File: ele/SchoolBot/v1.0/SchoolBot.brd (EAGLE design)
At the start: 100.1 x 58.3 mm, 56 parts, among them X1 M8, X2 M8, X4 POWER_IN

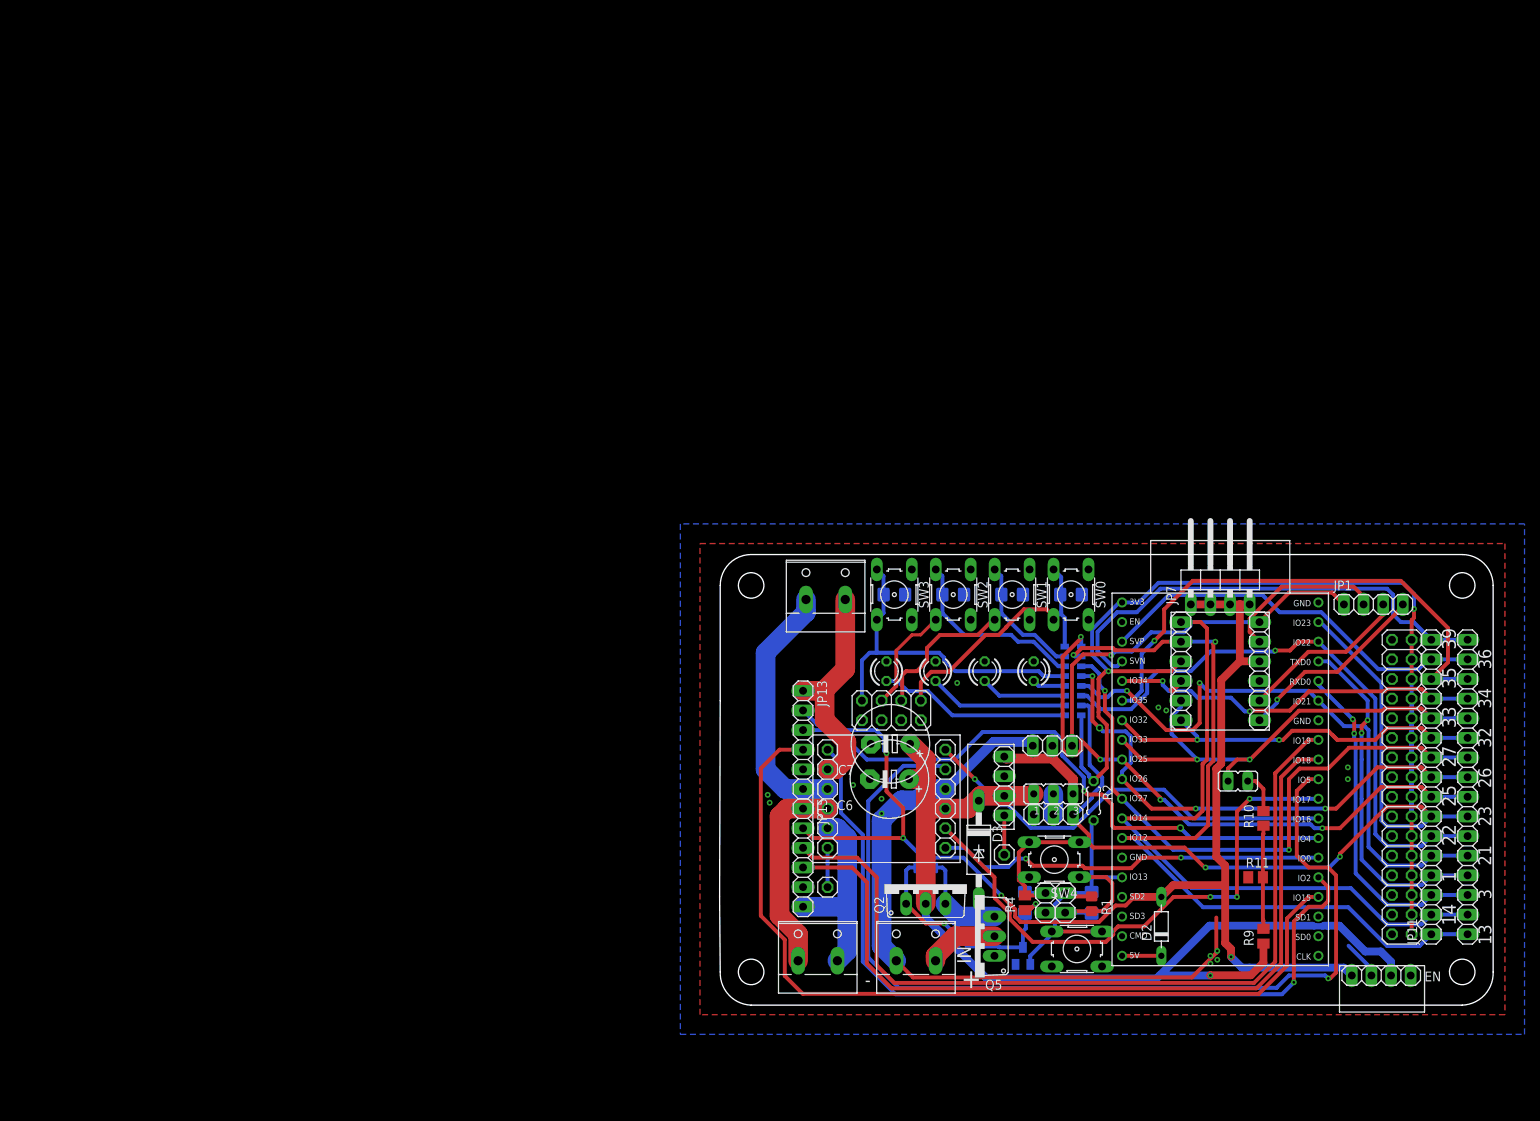
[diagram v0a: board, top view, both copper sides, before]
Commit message: new board
-komplenti prekreslini desky
-doplneni rady pinhedu gnd pro 5v piniste
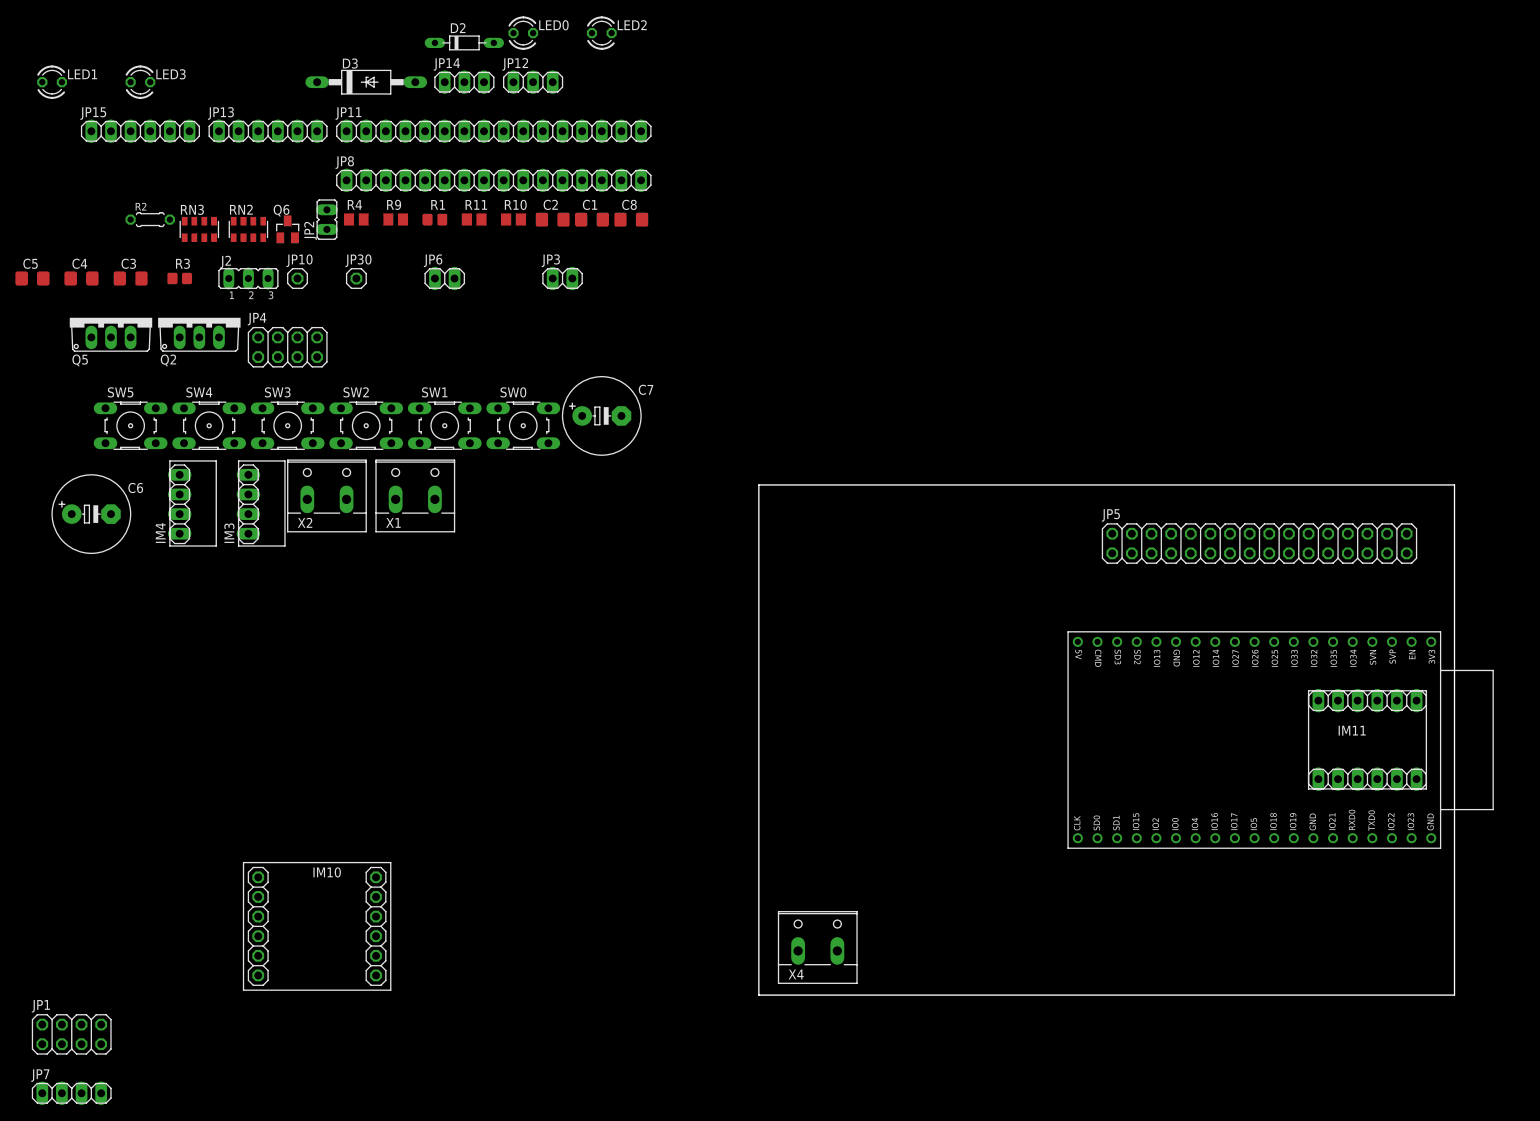
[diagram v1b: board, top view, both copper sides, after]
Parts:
- JP1: device pinhead:1X04 -> pinhead:2X04
- JP7: device pinhead:1X04/90 -> pinhead:1X04
- moved JP1 177.4 mm to (-88.9, -5.08)
- moved JP7 163.0 mm to (-88.9, -12.7)
- moved IM3 152.8 mm to (-67.3, 58.4), turned to 0 degrees
- moved JP8 148.4 mm to (-34.3, 105.4), turned to 0 degrees
- moved JP11 148.0 mm to (-34.3, 111.8), turned to 0 degrees
- moved R9 145.6 mm to (-47.0, 100.3), turned to 0 degrees
- moved D2 145.6 mm to (-38.1, 123.2), turned to 0 degrees
- moved R2 143.3 mm to (-78.7, 100.3), turned to 0 degrees
- moved LED1 142.7 mm to (-91.4, 118.1), turned to 0 degrees
- moved C5 140.5 mm to (-94.0, 92.7), flipped to the top
- moved SW5 139.9 mm to (-81.3, 73.7), turned to 0 degrees
- moved JP2 138.4 mm to (-55.9, 100.3), turned to 0 degrees
- moved Q5 137.4 mm to (-83.8, 87.6), turned to 0 degrees
- moved Q6 133.7 mm to (-61.0, 99.1), flipped to the top
- moved R11 132.1 mm to (-36.8, 100.3)
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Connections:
- net GND: now also JP1.2, JP1.4, JP1.6, JP1.8
- net GPIO13-5V: now also JP1.3; no longer JP1.2
- net GPIO32_5V: now also JP1.7; no longer JP1.4
- net GPIO33_5V: now also JP1.5; no longer JP1.3
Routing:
- net +3V3: track 189.8 -> 0.00 mm, vias 2 -> 0
- net +5V: track 162.6 -> 0.00 mm, vias 4 -> 0
- net VCC: track 133.4 -> 0.00 mm, vias 1 -> 0
- net PWM2: track 126.1 -> 0.00 mm, vias 1 -> 0
- net GND: track 117.8 -> 0.00 mm, vias 14 -> 0
- net ENC_B1: track 113.4 -> 0.00 mm
- net GPIO23: track 112.8 -> 0.00 mm, vias 2 -> 0
- net ENC_B2: track 107.9 -> 0.00 mm
- net GPIO12: track 107.5 -> 0.00 mm, vias 2 -> 0
- net ENC_A2: track 105.7 -> 0.00 mm
- net SLEEP: track 104.5 -> 0.00 mm, vias 1 -> 0
- net GPIO14: track 89.3 -> 0.00 mm
- net ENC_A1: track 79.2 -> 0.00 mm, vias 2 -> 0
- net GPIO27: track 78.9 -> 0.00 mm, vias 2 -> 0
- net GPIO25: track 78.8 -> 0.00 mm, vias 4 -> 0
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- removed copper zone on layer 1, net GND
- removed copper zone on layer 16, net GND
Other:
- board size 100.1 x 58.3 mm -> 90 x 66 mm
- board text removed: "+"
- board text removed: "-"
- board text removed: "1"
- board text removed: "13"
- board text removed: "14"
- board text removed: "21"
- board text removed: "22"
- board text removed: "23"
- board text removed: "25"
- board text removed: "26"
- board text removed: "27"
- board text removed: "3"
- board text removed: "3.3V"
- board text removed: "32"
- board text removed: "33"
- board text removed: "34"
- board text removed: "35"
- board text removed: "36"
- board text removed: "39"
- board text removed: "3V"
- board text removed: "5V"
- board text removed: "BLUE"
- board text removed: "Battery"
- board text removed: "C1"
- board text removed: "C2"
- board text removed: "EN"
- board text removed: "ENC_A1"
- board text removed: "ENC_A2"
- board text removed: "ENC_B1"
- board text removed: "ENC_B2"
- board text removed: "GND"
- board text removed: "GPIO13"
- board text removed: "GPIO15"
- board text removed: "GREEN"
- board text removed: "IN"
- board text removed: "IO13"
- board text removed: "IO14"
- board text removed: "IO15"
- board text removed: "IO32"
- board text removed: "IO33"
- board text removed: "M1"
- board text removed: "M2"
- board text removed: "MA1"
- board text removed: "MA2"
- board text removed: "MB1"
- board text removed: "MB2"
- board text removed: "OFF"
- board text removed: "ON"
- board text removed: "OUT1"
- board text removed: "OUT2"
- board text removed: "OUT3"
- board text removed: "OUT4"
- board text removed: "P-LED"
- board text removed: "PWM0"
- board text removed: "PWM1"
- board text removed: "PWM2"
- board text removed: "PWM3"
- board text removed: "RB3202-SchoolBot v0.1"
- board text removed: "RED"
- board text removed: "RX"
- board text removed: "S-leds"
- board text removed: "S-servo"
- board text removed: "SLEEP"
- board text removed: "SW0"
- board text removed: "SW1"
- board text removed: "SW2"
- board text removed: "SW3"
- board text removed: "ServoS-5V"
- board text removed: "TX"
- board text removed: "ULT"
- board text removed: "V5"
- board text removed: "VCC"

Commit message: nove rozlozeni
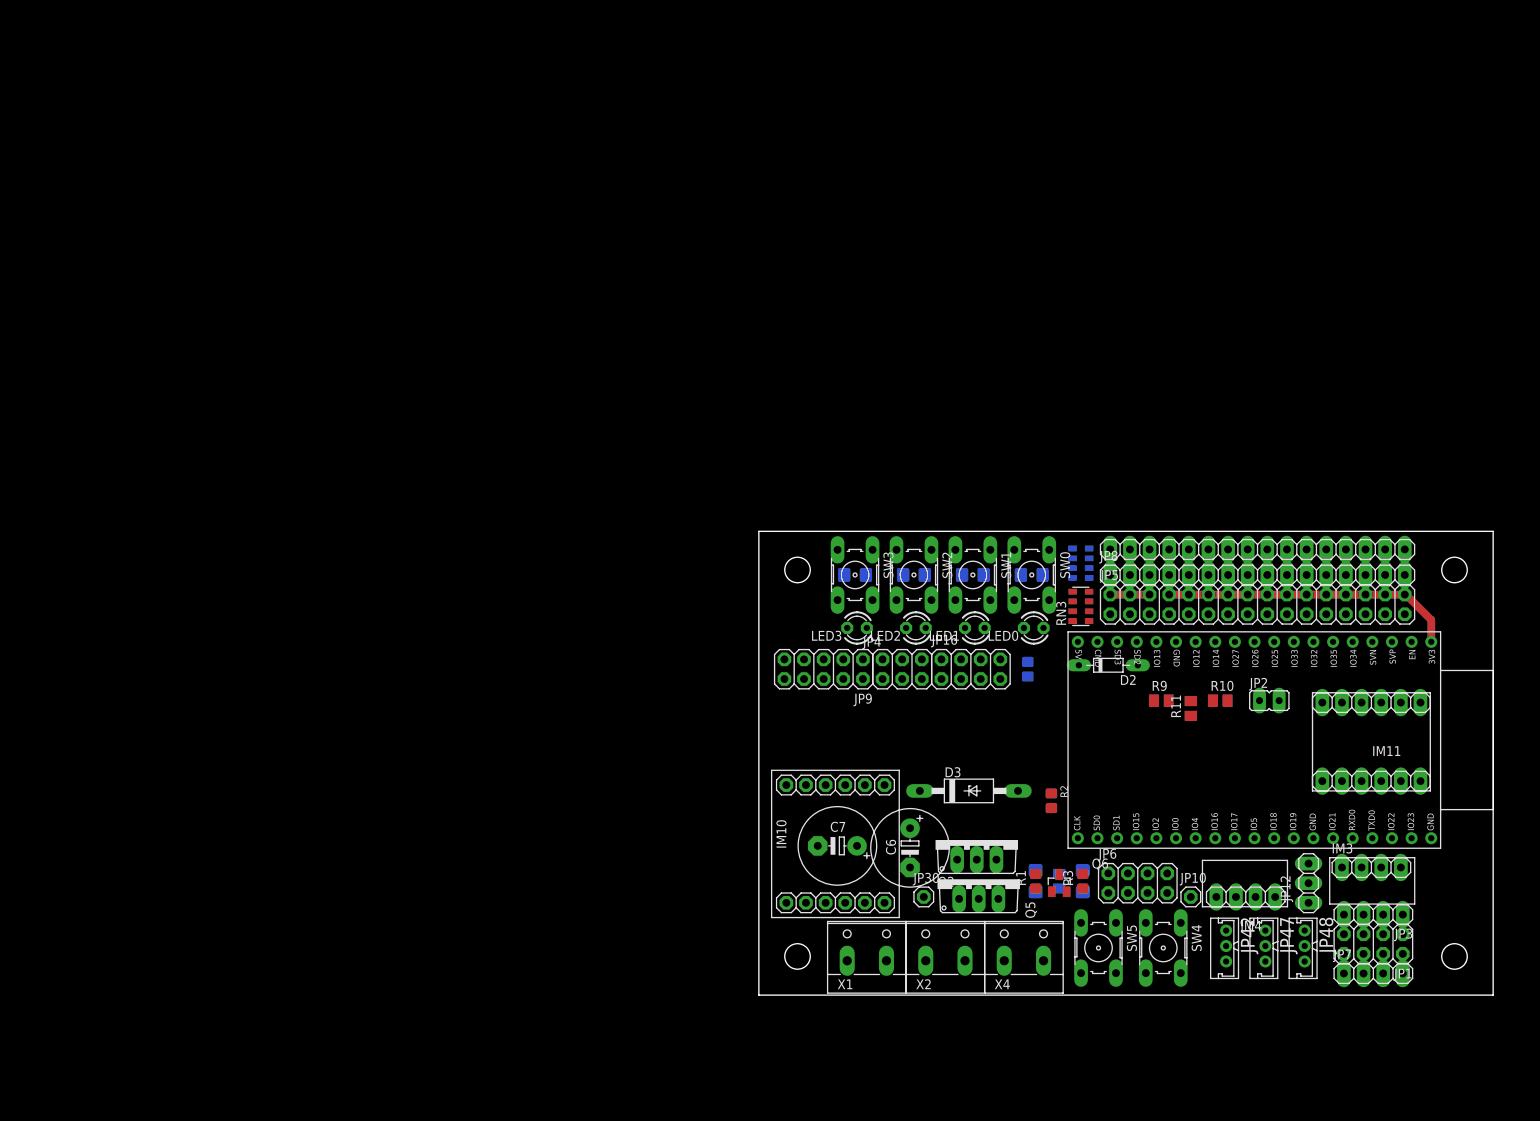
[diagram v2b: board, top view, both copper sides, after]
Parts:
- removed J2: (no value), jumper:JP2
- removed JP13, JP15: (no value), pinhead:1X06
- removed JP14: (no value), pinhead:1X03
- added JP16: (no value), pinhead:2X04
- added JP42, JP47, JP48: 292161-3, iServo_connector:292161-3
- added JP9: (no value), pinhead:2X05
- added R8: 10k, rcl_upravena:R0805
- JP3: value START_BUTTON -> (none); device pinhead:1X02 -> pinhead:1X04
- JP4: device pinhead:2X04 -> pinhead:2X03
- JP6: value STOP_BUTTON -> (none); device pinhead:1X02 -> pinhead:2X04
- R2: device rcl_upravena:0204/5 -> rcl_upravena:R0805
- moved JP7 169.1 mm to (79.5, 2.79)
- moved JP1 168.8 mm to (79.5, 6.60), turned to 180 degrees
- moved IM4 151.7 mm to (68.1, 11.4), turned to 90 degrees
- moved IM3 147.2 mm to (74.2, 17.8), turned to 270 degrees
- moved JP12 144.2 mm to (71.1, 14.5), turned to 90 degrees
- moved SW5 142.3 mm to (43.9, 6.10), turned to 270 degrees
- moved SW4 140.7 mm to (52.3, 6.10), turned to 270 degrees
- moved JP10 140.6 mm to (55.9, 12.7)
- moved R3 140.5 mm to (41.9, 14.7), turned to 90 degrees
- moved R2 138.7 mm to (37.8, 25.1), turned to 270 degrees
- moved LED1 138.7 mm to (27.9, 47.5), turned to 180 degrees
- moved JP2 136.9 mm to (66.0, 38.1), turned to 270 degrees
- moved C5 134.9 mm to (35.3, 54.4), flipped to the bottom
- moved Q5 133.7 mm to (28.4, 15.0)
- moved JP3 133.3 mm to (79.5, 10.4), turned to 180 degrees
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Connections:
- net BAT_PROT1 renamed BAT_POL+
- removed net N$3: J2.2, JP14.2
- removed net START_BUTTON1: C1.2, JP3.1, R4.2, SW4.3, SW4.4
- new net EN: JP16.4, R8.1
- new net N$5: JP9.10, JP9.2, JP9.4, JP9.6, JP9.8
- new net N$7: C1.2, JP16.6, R4.2, SW4.3, SW4.4
- net +3V3: now also R8.2
- net +5V: now also JP1.2, JP1.4, JP1.6, JP1.8, JP16.2, JP6.1, JP6.2; no longer JP13.2, JP15.2, JP7.1, JP7.2, JP7.3, JP7.4
- net ENC_A1: now also JP6.6; no longer JP13.3
- net ENC_A2: now also JP6.3; no longer JP15.4
- net ENC_B1: now also JP6.4; no longer JP13.4
- net ENC_B2: now also JP6.5; no longer JP15.3
- net GND: now also JP16.1, JP16.3, JP16.5, JP16.7, JP42.1, JP47.1, JP48.1, JP6.7, JP6.8, JP7.1, JP7.2, JP7.3, JP7.4; no longer JP1.2, JP1.4, JP1.6, JP1.8, JP13.5, JP14.1, JP15.5, JP3.2, JP4.7, JP6.2
- net GPIO13-5V: now also JP3.2
- net GPIO14-5V: now also JP3.1
- net GPIO23: now also JP42.3, JP47.3, JP48.3; no longer JP14.3
- net GPIO32_5V: now also JP3.4
- net GPIO33_5V: now also JP3.3
- net LED0: now also JP9.1
- net LED1: now also JP9.3
- net LED2: now also JP9.5
- net LED3: now also JP9.7
- net M1A: now also X1.1; no longer JP13.1, X1.2
- net M1B: now also X1.2; no longer JP13.6, X1.1
- net M2A: no longer JP15.1
- net M2B: no longer JP15.6
- net OFF: now also JP16.8; no longer JP6.1
- net SERVO_STEPDOWN_5V: no longer J2.3
- net SW0: now also JP4.6; no longer JP4.8
- net SW1: now also JP4.4; no longer JP4.6
- net SW2: now also JP4.2; no longer JP4.4
- net SW3: now also JP9.9; no longer JP4.2
- net VCC: now also JP42.2, JP47.2, JP48.2; no longer J2.1
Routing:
- net +3V3: track 0.00 -> 43.2 mm
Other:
- board size 90 x 66 mm -> 95 x 60 mm
